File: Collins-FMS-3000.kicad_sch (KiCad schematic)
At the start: 26 parts, among them J3 TC2030-IDC-NL, U2 TCA8418, U4 IS31FL3733B

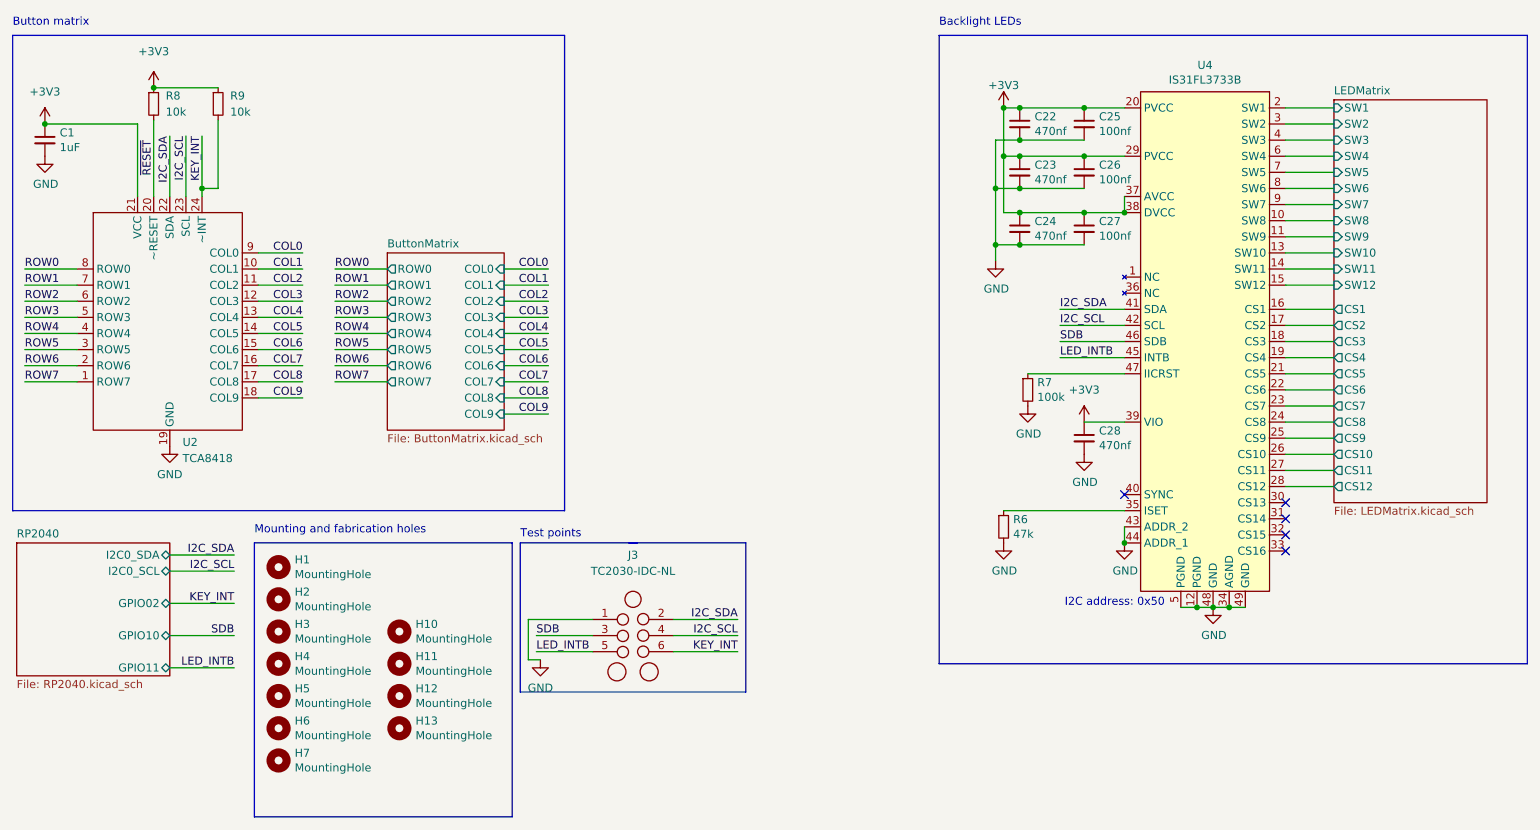
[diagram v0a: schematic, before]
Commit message: FULLY ROUTED
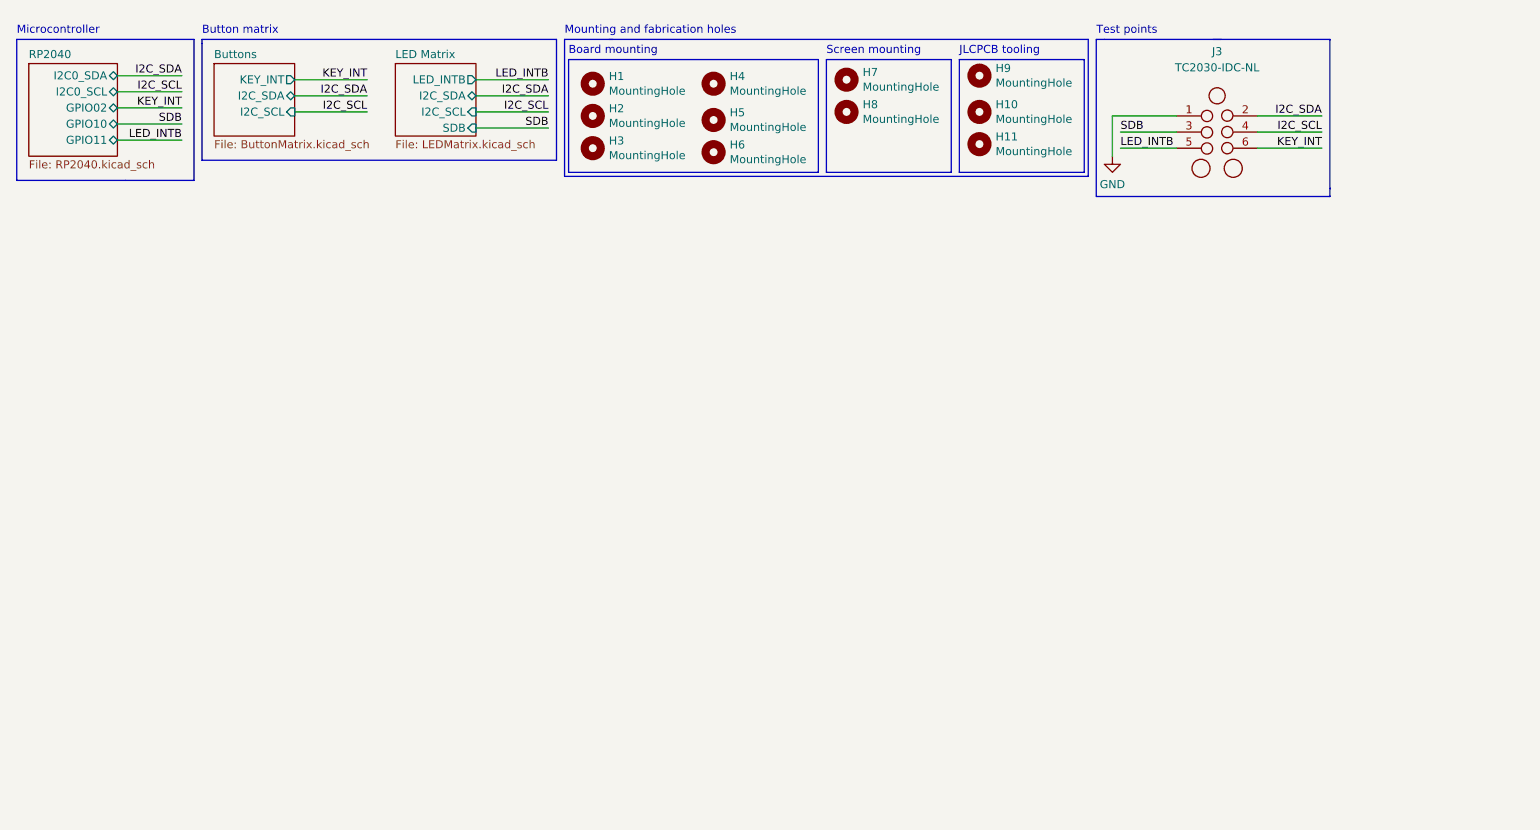
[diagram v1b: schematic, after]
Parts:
- removed C1: 1uF, Custom_Footprints:Perfect_0402, symbol Device:C_Small
- removed C22, C23, C24, C28: 470nf, Custom_Footprints:Perfect_0402, symbol Device:C_Small
- removed C25, C26, C27: 100nf, Custom_Footprints:Perfect_0402, symbol Device:C_Small
- removed H4: MountingHole, MountingHole:MountingHole_3.2mm_M3, symbol Mechanical:MountingHole
- removed H5, H6: MountingHole, Collins-FMS-3000:JLCPCB_Tooling_Hole, symbol Mechanical:MountingHole
- removed R6: 47k, Custom_Footprints:Perfect_0402, symbol Device:R_Small
- removed R7: 100k, Resistor_SMD:R_0603_1608Metric, symbol Device:R_Small
- removed R8, R9: 10k, Custom_Footprints:Perfect_0402, symbol Device:R_Small
- removed U2: TCA8418, Package_DFN_QFN:WQFN-24-1EP_4x4mm_P0.5mm_EP2.6x2.6mm, symbol Custom_Symbols:TCA8418
- removed U4: IS31FL3733B, Package_QFP:TQFP-48-1EP_7x7mm_P0.5mm_EP5x5mm_ThermalVias, symbol Collins-FMS-3000:IS31FL3733B
- added H7, H8: MountingHole, MountingHole:MountingHole_3.2mm_M3, symbol Mechanical:MountingHole
- added H9: MountingHole, Collins-FMS-3000:JLCPCB_Tooling_Hole, symbol Mechanical:MountingHole
- H11: renamed from H13; footprint MountingHole:MountingHole_3.2mm_M3 -> Collins-FMS-3000:JLCPCB_Tooling_Hole
- renumbered H7 to H10, H10 to H4, H11 to H5, H12 to H6
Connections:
- no-connect marks 5 -> 0
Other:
- sheet ButtonMatrix renamed Buttons
- sheet LEDMatrix renamed LED Matrix
- sheet Buttons ports: added I2C_SCL, I2C_SDA, KEY_INT; removed COL0, COL1, COL2, COL3, COL4, COL5, COL6, COL7, COL8, COL9, ROW0, ROW1, ROW2, ROW3, ROW4, ROW5, ROW6, ROW7
- sheet LED Matrix ports: added I2C_SCL, I2C_SDA, LED_INTB, SDB; removed CS1, CS10, CS11, CS12, CS2, CS3, CS4, CS5, CS6, CS7, CS8, CS9, SW1, SW10, SW11, SW12, SW2, SW3, SW4, SW5, SW6, SW7, SW8, SW9
- note added: "Board mounting"
- note added: "JLCPCB tooling"
- note added: "Microcontroller"
- note added: "Screen mounting"
- note removed: "Backlight LEDs"
- note removed: "I2C address: 0x50"
- moved on the sheet: H1, H10, H11, H2, H3, H4, H5, H6, J3
